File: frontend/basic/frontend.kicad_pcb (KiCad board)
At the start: 2 copper layers, 24.6 x 49.9 mm, 16 parts, among them CN1 EDGE, J1 J1, J2 J2, P1 BNC, P2 BNC, T1 TRANSF, T2 TRANSF

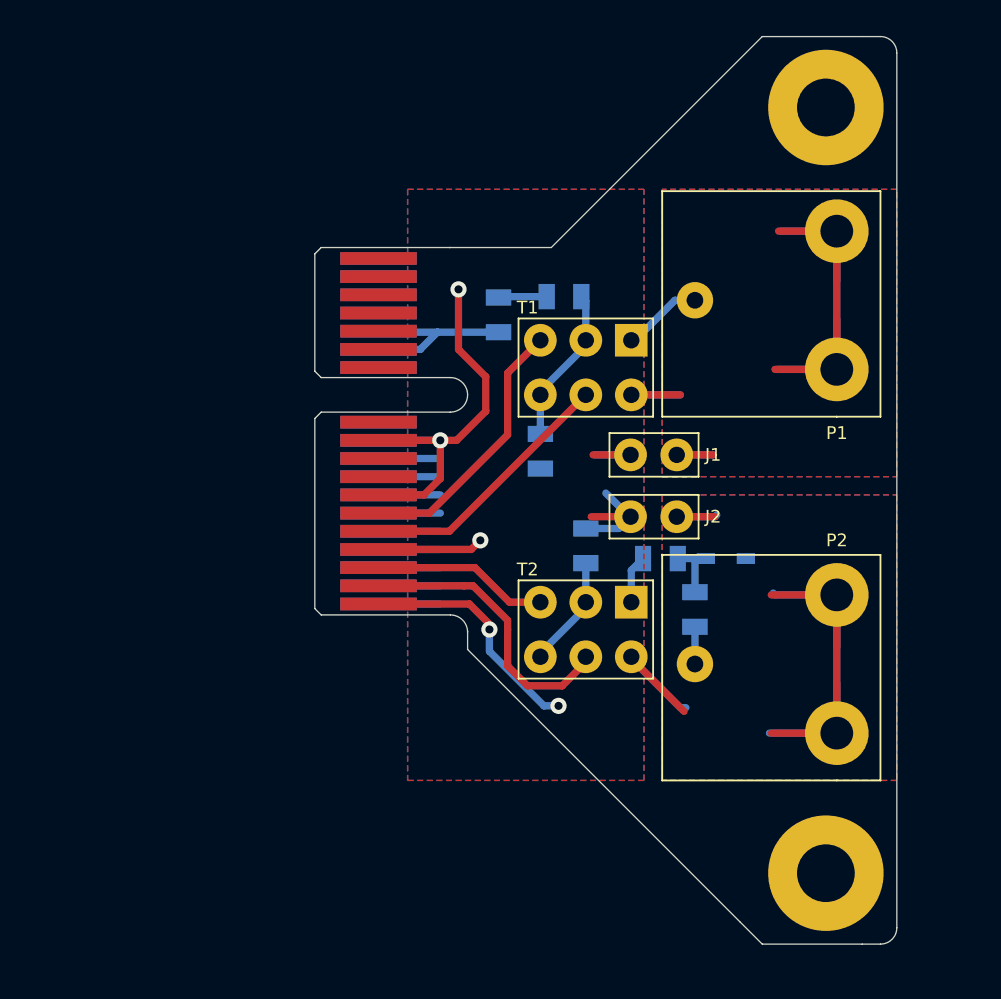
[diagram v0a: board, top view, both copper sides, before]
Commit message: Updated basic frontend
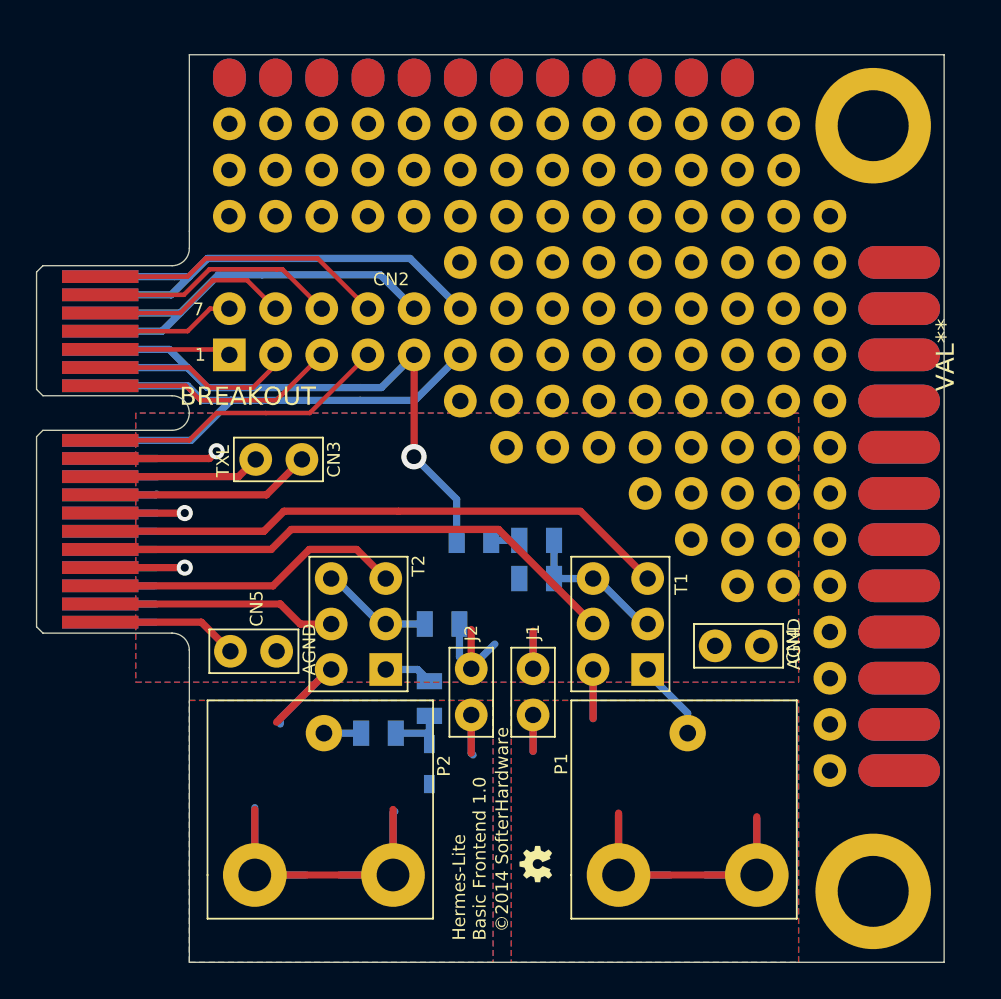
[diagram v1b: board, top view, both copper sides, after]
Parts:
- added CN2: BREAKOUT, HERMESLITE:BREAKOUT, F.Cu at (101.6, 88.9)
- added CN3: TXL, HERMESLITE:JUMPER, F.Cu at (103.0, 94.7)
- added CN4: AGND, HERMESLITE:JUMPER, F.Cu at (130.8, 104.9)
- added CN5: AGND, HERMESLITE:JUMPER, F.Cu at (104.2, 105.2)
- added G***: OSHW-logo_silkscreen-front_2mm, OSHW:OSHW-logo_silkscreen-front_2mm, F.Cu at (118.5, 116.9)
- added G***: OSHW-logo_silkscreen-front_2mm, OSHW:OSHW-logo_silkscreen-front_2mm, B.Cu at (118.7, 113.7)
- added HOLE: VAL**, HERMESLITE:HOLE, F.Cu at (101.6, 81.3)
- added HOLE: VAL**, HERMESLITE:HOLE, F.Cu at (109.2, 76.2)
- added HOLE: VAL**, HERMESLITE:HOLE, F.Cu at (109.2, 78.7)
- added HOLE: VAL**, HERMESLITE:HOLE, F.Cu at (109.2, 81.3)
- added HOLE: VAL**, HERMESLITE:HOLE, F.Cu at (111.8, 81.3)
- added HOLE: VAL**, HERMESLITE:HOLE, F.Cu at (114.3, 81.3)
- added HOLE: VAL**, HERMESLITE:HOLE, F.Cu at (116.8, 81.3)
- added HOLE: VAL**, HERMESLITE:HOLE, F.Cu at (119.4, 81.3)
- added HOLE: VAL**, HERMESLITE:HOLE, F.Cu at (121.9, 81.3)
- added HOLE: VAL**, HERMESLITE:HOLE, F.Cu at (124.5, 81.3)
- added HOLE: VAL**, HERMESLITE:HOLE, F.Cu at (127.0, 81.3)
- added HOLE: VAL**, HERMESLITE:HOLE, F.Cu at (101.6, 78.7)
- added HOLE: VAL**, HERMESLITE:HOLE, F.Cu at (129.5, 81.3)
- added HOLE: VAL**, HERMESLITE:HOLE, F.Cu at (132.1, 81.3)
- added HOLE: VAL**, HERMESLITE:HOLE, F.Cu at (132.1, 78.7)
- added HOLE: VAL**, HERMESLITE:HOLE, F.Cu at (132.1, 76.2)
- added HOLE: VAL**, HERMESLITE:HOLE, F.Cu at (129.5, 76.2)
- added HOLE: VAL**, HERMESLITE:HOLE, F.Cu at (127.0, 76.2)
- added HOLE: VAL**, HERMESLITE:HOLE, F.Cu at (124.5, 76.2)
- added HOLE: VAL**, HERMESLITE:HOLE, F.Cu at (121.9, 76.2)
- added HOLE: VAL**, HERMESLITE:HOLE, F.Cu at (119.4, 76.2)
- added HOLE: VAL**, HERMESLITE:HOLE, F.Cu at (116.8, 76.2)
- added HOLE: VAL**, HERMESLITE:HOLE, F.Cu at (101.6, 76.2)
- added HOLE: VAL**, HERMESLITE:HOLE, F.Cu at (114.3, 76.2)
- added HOLE: VAL**, HERMESLITE:HOLE, F.Cu at (111.8, 76.2)
- added HOLE: VAL**, HERMESLITE:HOLE, F.Cu at (116.8, 83.8)
- added HOLE: VAL**, HERMESLITE:HOLE, F.Cu at (114.3, 83.8)
- added HOLE: VAL**, HERMESLITE:HOLE, F.Cu at (111.8, 78.7)
- added HOLE: VAL**, HERMESLITE:HOLE, F.Cu at (114.3, 78.7)
- added HOLE: VAL**, HERMESLITE:HOLE, F.Cu at (116.8, 78.7)
- added HOLE: VAL**, HERMESLITE:HOLE, F.Cu at (119.4, 78.7)
- added HOLE: VAL**, HERMESLITE:HOLE, F.Cu at (121.9, 78.7)
- added HOLE: VAL**, HERMESLITE:HOLE, F.Cu at (124.5, 78.7)
- added HOLE: VAL**, HERMESLITE:HOLE, F.Cu at (104.1, 81.3)
- added HOLE: VAL**, HERMESLITE:HOLE, F.Cu at (127.0, 78.7)
- added HOLE: VAL**, HERMESLITE:HOLE, F.Cu at (129.5, 78.7)
- added HOLE: VAL**, HERMESLITE:HOLE, F.Cu at (119.4, 83.8)
- added HOLE: VAL**, HERMESLITE:HOLE, F.Cu at (121.9, 83.8)
- added HOLE: VAL**, HERMESLITE:HOLE, F.Cu at (124.5, 83.8)
- added HOLE: VAL**, HERMESLITE:HOLE, F.Cu at (127.0, 83.8)
- added HOLE: VAL**, HERMESLITE:HOLE, F.Cu at (129.5, 83.8)
- added HOLE: VAL**, HERMESLITE:HOLE, F.Cu at (132.1, 83.8)
- added HOLE: VAL**, HERMESLITE:HOLE, F.Cu at (132.1, 86.4)
- added HOLE: VAL**, HERMESLITE:HOLE, F.Cu at (129.5, 86.4)
- added HOLE: VAL**, HERMESLITE:HOLE, F.Cu at (104.1, 78.7)
- added HOLE: VAL**, HERMESLITE:HOLE, F.Cu at (127.0, 86.4)
- added HOLE: VAL**, HERMESLITE:HOLE, F.Cu at (124.5, 86.4)
- added HOLE: VAL**, HERMESLITE:HOLE, F.Cu at (121.9, 86.4)
- added HOLE: VAL**, HERMESLITE:HOLE, F.Cu at (119.4, 86.4)
- added HOLE: VAL**, HERMESLITE:HOLE, F.Cu at (116.8, 86.4)
- added HOLE: VAL**, HERMESLITE:HOLE, F.Cu at (116.8, 88.9)
- added HOLE: VAL**, HERMESLITE:HOLE, F.Cu at (119.4, 88.9)
- added HOLE: VAL**, HERMESLITE:HOLE, F.Cu at (121.9, 88.9)
- added HOLE: VAL**, HERMESLITE:HOLE, F.Cu at (124.5, 88.9)
- added HOLE: VAL**, HERMESLITE:HOLE, F.Cu at (127.0, 88.9)
- added HOLE: VAL**, HERMESLITE:HOLE, F.Cu at (104.1, 76.2)
- added HOLE: VAL**, HERMESLITE:HOLE, F.Cu at (129.5, 88.9)
- added HOLE: VAL**, HERMESLITE:HOLE, F.Cu at (132.1, 88.9)
- added HOLE: VAL**, HERMESLITE:HOLE, F.Cu at (132.1, 91.4)
- added HOLE: VAL**, HERMESLITE:HOLE, F.Cu at (129.5, 91.4)
- added HOLE: VAL**, HERMESLITE:HOLE, F.Cu at (127.0, 91.4)
- added HOLE: VAL**, HERMESLITE:HOLE, F.Cu at (124.5, 91.4)
- added HOLE: VAL**, HERMESLITE:HOLE, F.Cu at (121.9, 91.4)
- added HOLE: VAL**, HERMESLITE:HOLE, F.Cu at (119.4, 91.4)
- added HOLE: VAL**, HERMESLITE:HOLE, F.Cu at (116.8, 91.4)
- added HOLE: VAL**, HERMESLITE:HOLE, F.Cu at (114.3, 91.4)
- added HOLE: VAL**, HERMESLITE:HOLE, F.Cu at (106.7, 81.3)
- added HOLE: VAL**, HERMESLITE:HOLE, F.Cu at (134.6, 81.3)
- added HOLE: VAL**, HERMESLITE:HOLE, F.Cu at (134.6, 83.8)
- added HOLE: VAL**, HERMESLITE:HOLE, F.Cu at (134.6, 86.4)
- added HOLE: VAL**, HERMESLITE:HOLE, F.Cu at (134.6, 88.9)
- added HOLE: VAL**, HERMESLITE:HOLE, F.Cu at (134.6, 91.4)
- added HOLE: VAL**, HERMESLITE:HOLE, F.Cu at (116.8, 94.0)
- added HOLE: VAL**, HERMESLITE:HOLE, F.Cu at (119.4, 94.0)
- added HOLE: VAL**, HERMESLITE:HOLE, F.Cu at (121.9, 94.0)
- added HOLE: VAL**, HERMESLITE:HOLE, F.Cu at (124.5, 94.0)
- added HOLE: VAL**, HERMESLITE:HOLE, F.Cu at (127.0, 94.0)
- added HOLE: VAL**, HERMESLITE:HOLE, F.Cu at (106.7, 78.7)
- added HOLE: VAL**, HERMESLITE:HOLE, F.Cu at (129.5, 94.0)
- added HOLE: VAL**, HERMESLITE:HOLE, F.Cu at (132.1, 94.0)
- added HOLE: VAL**, HERMESLITE:HOLE, F.Cu at (134.6, 94.0)
- added HOLE: VAL**, HERMESLITE:HOLE, F.Cu at (124.5, 96.5)
- added HOLE: VAL**, HERMESLITE:HOLE, F.Cu at (127.0, 96.5)
- added HOLE: VAL**, HERMESLITE:HOLE, F.Cu at (129.5, 96.5)
- added HOLE: VAL**, HERMESLITE:HOLE, F.Cu at (132.1, 96.5)
- added HOLE: VAL**, HERMESLITE:HOLE, F.Cu at (134.6, 96.5)
- added HOLE: VAL**, HERMESLITE:HOLE, F.Cu at (127.0, 99.1)
- added HOLE: VAL**, HERMESLITE:HOLE, F.Cu at (129.5, 99.1)
- added HOLE: VAL**, HERMESLITE:HOLE, F.Cu at (106.7, 76.2)
- added HOLE: VAL**, HERMESLITE:HOLE, F.Cu at (132.1, 99.1)
- added HOLE: VAL**, HERMESLITE:HOLE, F.Cu at (134.6, 99.1)
- added HOLE: VAL**, HERMESLITE:HOLE, F.Cu at (129.5, 101.6)
- added HOLE: VAL**, HERMESLITE:HOLE, F.Cu at (132.1, 101.6)
- added HOLE: VAL**, HERMESLITE:HOLE, F.Cu at (134.6, 101.6)
- added HOLE: VAL**, HERMESLITE:HOLE, F.Cu at (134.6, 104.1)
- added HOLE: VAL**, HERMESLITE:HOLE, F.Cu at (134.6, 106.7)
- added HOLE: VAL**, HERMESLITE:HOLE, F.Cu at (134.6, 109.2)
- added HOLE: VAL**, HERMESLITE:HOLE, F.Cu at (134.6, 111.8)
- added PROTOEDGE12L: VAL**, HERMESLITE:PROTOEDGE12L, F.Cu at (138.4, 111.8)
- added PROTOEDGE12S: VAL**, HERMESLITE:PROTOEDGE12S, F.Cu at (101.6, 73.7)
- J1: value J1 -> 0
- J2: value J2 -> 0
- T1: value TRANSF -> 4:1
- T2: value TRANSF -> 8:1
- moved P1 32.6 mm to (126.8, 117.5), turned to 0 degrees
- moved P2 30.5 mm to (106.8, 117.5), turned to 0 degrees
- moved D1 19.8 mm to (112.6, 111.4), turned to 270 degrees
- moved C4 18.7 mm to (109.8, 109.7), turned to 0 degrees
- moved T2 16.5 mm to (107.2, 106.2), turned to 0 degrees
- moved J1 16.3 mm to (118.3, 108.7), turned to 0 degrees
- moved J2 15.7 mm to (114.9, 108.7), turned to 0 degrees
- moved CN1 15.3 mm to (91.0, 92.1)
- moved T1 15.2 mm to (121.6, 106.2), turned to 0 degrees
- moved C3 14.9 mm to (112.6, 107.8), turned to 90 degrees
- moved R1 13.5 mm to (118.5, 99.1)
- moved FB1 12.5 mm to (115.0, 99.1), turned to 0 degrees
- moved C2 8.99 mm to (113.3, 103.7), turned to 0 degrees
- moved C1 7.00 mm to (118.5, 101.2), turned to 180 degrees
- moved MH 1.49 mm to (135.5, 76.3)
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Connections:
- CN1 pad A12: Net-(CN1-PadA12) -> Net-(CN1-PadA11)
- CN1 pad A16: Net-(CN1-PadA16) -> Net-(CN1-PadA15)
- CN1 pad A18: Net-(CN1-PadA18) -> Net-(CN1-PadA17)
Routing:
- net Net-(CN1-PadA11): track 0.00 -> 29.3 mm
- net Net-(CN1-PadA17): track 0.00 -> 26.7 mm
- net Net-(CN1-PadA13): track 10.3 -> 34.9 mm, vias 0 -> 1
- net Net-(CN1-PadA15): track 0.00 -> 23.7 mm
- net GND: track 83.5 -> 65.5 mm, vias 5 -> 3
- net Net-(CN1-PadB6): track 14.8 -> 32.1 mm
- net Net-(CN1-PadB11): track 0.00 -> 16.7 mm
- net Net-(CN1-PadB18): track 0.00 -> 16.3 mm
- net Net-(CN1-PadB5): track 14.5 -> 29.7 mm
- net Net-(CN1-PadB17): track 0.00 -> 13.7 mm
- net Net-(CN1-PadB12): track 0.00 -> 13.5 mm
- net Net-(CN1-PadB8): track 0.00 -> 11.9 mm
- net Net-(CN1-PadB13): track 0.00 -> 11.2 mm
- net Net-(CN1-PadB16): track 0.00 -> 11.0 mm
- net Net-(CN1-PadB9): track 0.00 -> 8.94 mm
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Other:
- board size 24.6 x 49.9 mm -> 41.5 x 49.9 mm
- board text added: "Hermes-Lite Basic Frontend 1.0"
- board text removed: "Hermes-Lite Basic Frontend 0.9"

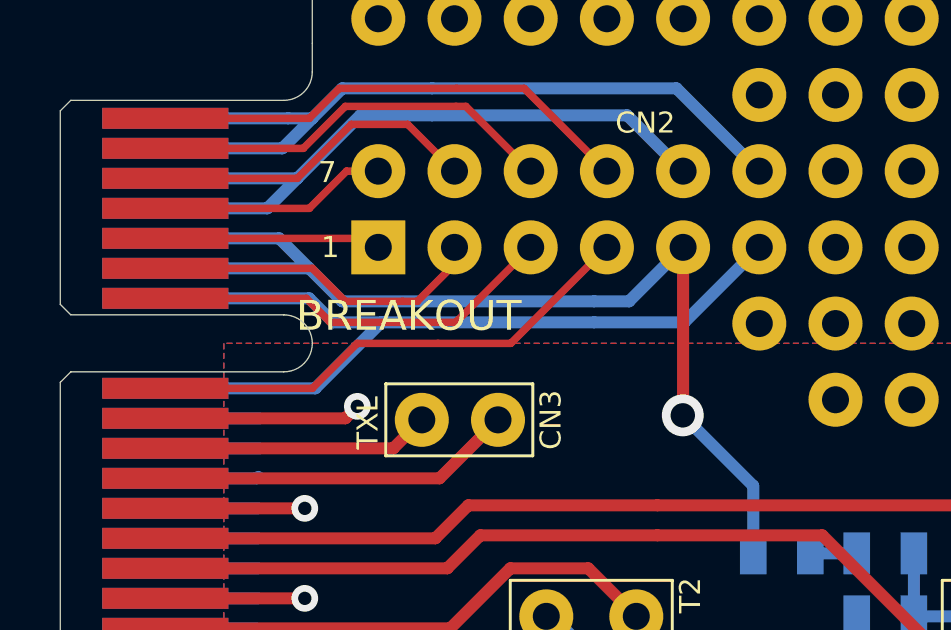
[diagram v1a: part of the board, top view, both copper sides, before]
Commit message: Added revision 1.21
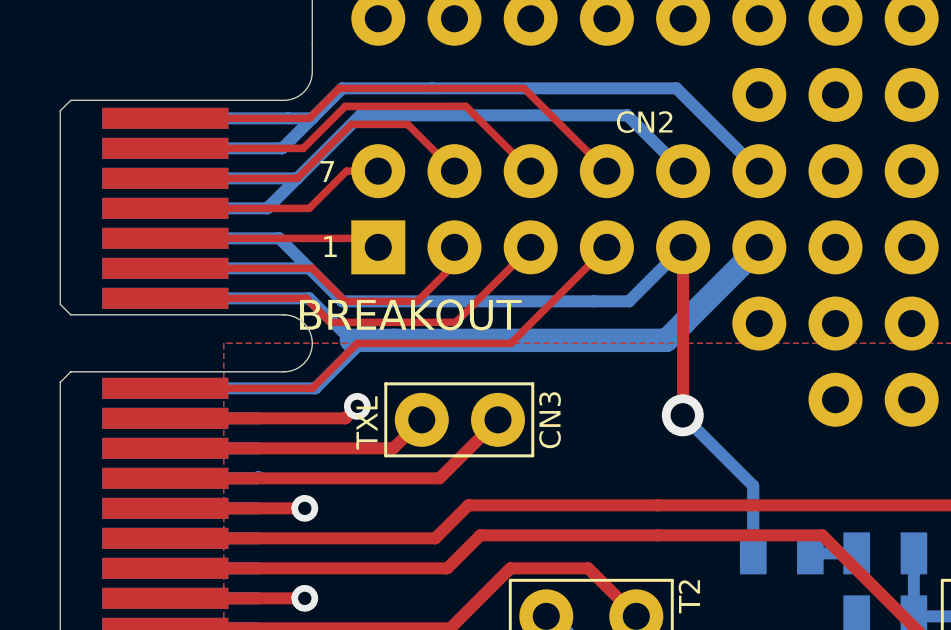
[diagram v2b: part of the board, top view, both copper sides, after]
